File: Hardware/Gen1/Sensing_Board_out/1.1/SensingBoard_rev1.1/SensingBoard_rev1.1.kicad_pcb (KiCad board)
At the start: 6 copper layers, 40 x 40 mm, 89 parts, among them J1 USB_C_Receptacle, J2 3221-10-0300-00, J3 F32R-1A7H1-11024, J5 RS1-02-G, J6 RS1-02-G, J7 RS1-02-G, J9 RS1-02-G, SW1 PTS815 SJM 250 SMTR LFS, SW2 PTS815 SJM 250 SMTR LFS, U2 BNO055, U3 MIC5504-3.3YM5, U4 FT232RQ, U5 MIC5504-1.8YM5, U6 MCP1700x-280xxTT, U7 ESP32-S3, U8 GD25D05CT, Y1 ABM8G-40.000MHZ-18-D2Y-T

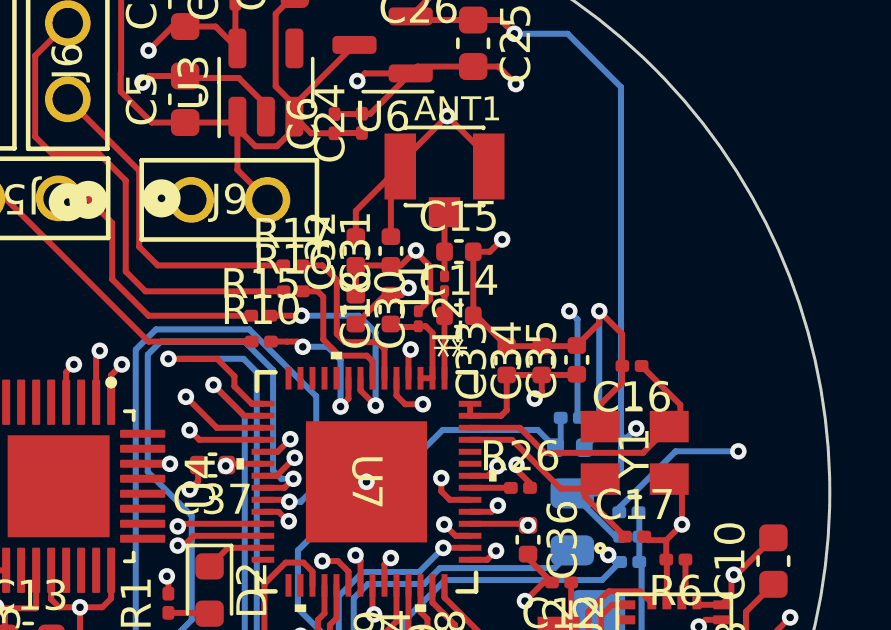
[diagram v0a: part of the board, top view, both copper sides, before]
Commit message: update
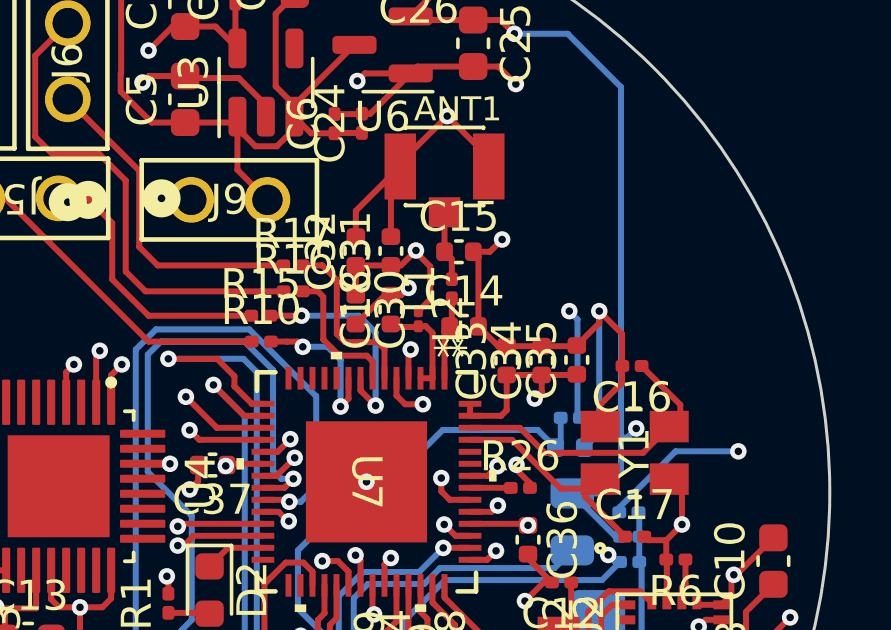
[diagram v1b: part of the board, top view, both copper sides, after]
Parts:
- L1: footprint Inductor_SMD:L_01005_0402Metric -> Inductor_SMD:L_0201_0603Metric
- moved C14 0.39 mm to (138.0, 56.9)
- moved L1 0.30 mm to (137.6, 55.7)

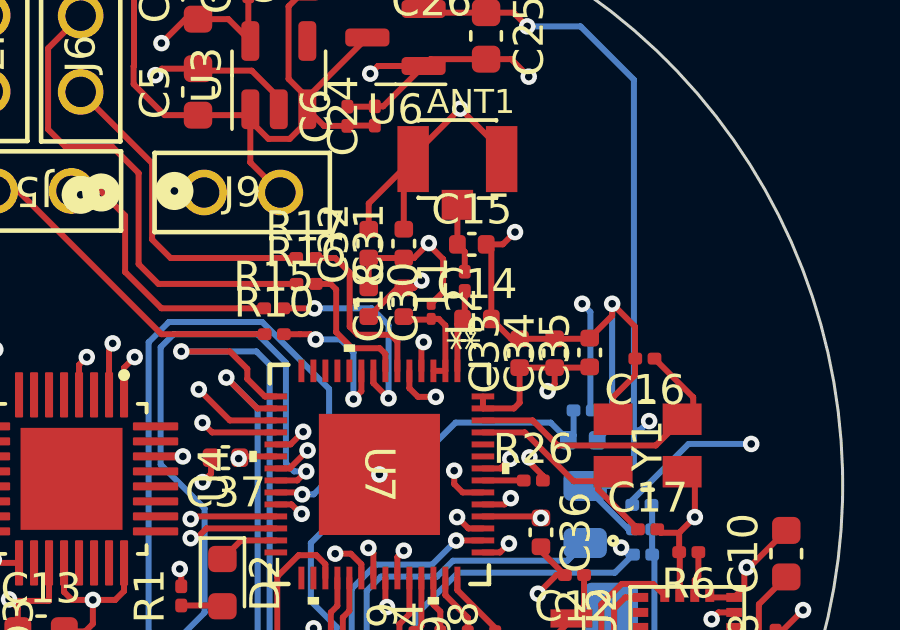
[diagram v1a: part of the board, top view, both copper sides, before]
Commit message: updates
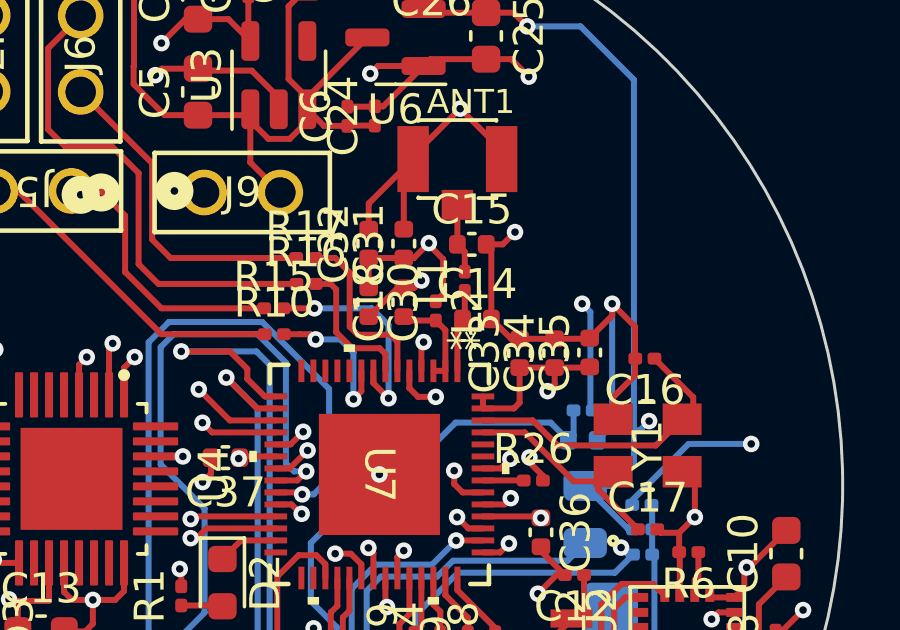
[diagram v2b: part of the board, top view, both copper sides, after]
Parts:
- L2: footprint Inductor_SMD:L_01005_0402Metric -> Inductor_SMD:L_0201_0603Metric
- moved L2 0.15 mm to (136.6, 56.7)
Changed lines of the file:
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@@
     (tags "ESP32-S3 ")
     (property "Mfr" "Espressif Systems")
-    (property "Mfr P/N" "ESP32-S3-WROOM-1-N8R2")
+    (property "Mfr P/N" "ESP32-S3R8")
     (property "Note" "")
     (property "Price" "4.3420")
-    (property "Purchase-URL" "https://www.lcsc.com/product-detail/WiFi-Modules_Espressif-Systems-ESP32-S3-WROOM-1-N8R2_C2913204.html")
+    (property "Purchase-URL" "https://www.lcsc.com/product-detail/RF-Transceiver-ICs_Espressif-Systems-ESP32-S3R8_C2913194.html")
     (property "Sheetfile" "SensingBoard_rev1.1.kicad_sch")
     (property "Sheetname" "")
     (property "Supplier 1" "LCSC")
-    (property "Supplier 1 P/N" "C2913204")
+    (property "Supplier 1 P/N" "C2913194")
     (property "ki_keywords" "ESP32-S3")
     (attr smd)
@@
         (effects (font (size 1 1) (thickness 0.15)))
     )
-    (fp_text user "*" (at -3.075001 -2.8 -90) (layer "F.Fab")
+    (fp_text user "*" (at -3.075001 -2.8 -90 unlocked) (layer "F.Fab")
         (effects (font (size 1 1) (thickness 0.15)))
     )
-    (fp_text user "*" (at -3.075001 -2.8 -90 unlocked) (layer "F.Fab")
+    (fp_text user "*" (at -3.075001 -2.8 -90) (layer "F.Fab")
         (effects (font (size 1 1) (thickness 0.15)))
     )
@@
     )
   )
-  (footprint "Inductor_SMD:L_01005_0402Metric" (layer "F.Cu")
-    (at 136.4488 56.6928 -90)
-    (descr "Inductor SMD 01005 (0402 Metric), square (rectangular) end terminal, IPC_7351 nominal, (Body size source: http://www.vishay.com/docs/20056/crcw01005e3.pdf), generated with kicad-footprint-generator")
+  (footprint "Inductor_SMD:L_0201_0603Metric" (layer "F.Cu")
+    (at 136.6012 56.6776 -90)
+    (descr "Inductor SMD 0201 (0603 Metric), square (rectangular) end terminal, IPC_7351 nominal, (Body size source: https://www.vishay.com/docs/20052/crcw0201e3.pdf), generated with kicad-footprint-generator")
     (tags "inductor")
     (property "Mfr" "Murata Electronics")
@@
     (property "ki_keywords" "inductor choke coil reactor magnetic")
     (attr smd)
-    (fp_text reference "L2" (at 0 -1 90) (layer "F.SilkS")
+    (fp_text reference "L2" (at 0 -1.05 -90) (layer "F.SilkS")
         (effects (font (size 1 1) (thickness 0.15)))
     )
-    (fp_text value "2nH" (at 0 1 90) (layer "F.Fab")
+    (fp_text value "2nH" (at 0 1.05 -90) (layer "F.Fab")
         (effects (font (size 1 1) (thickness 0.15)))
     )
-    (fp_text user "${REFERENCE}" (at 0 -0.62 90) (layer "F.Fab")
+    (fp_text user "${REFERENCE}" (at 0 -0.68 -90) (layer "F.Fab")
         (effects (font (size 0.25 0.25) (thickness 0.04)))
     )
-    (fp_line (start -0.6 -0.3) (end 0.6 -0.3)
+    (fp_line (start -0.7 -0.35) (end 0.7 -0.35)
       (stroke (width 0.05) (type solid)) (layer "F.CrtYd"))
-    (fp_line (start -0.6 0.3) (end -0.6 -0.3)
+    (fp_line (start -0.7 0.35) (end -0.7 -0.35)
       (stroke (width 0.05) (type solid)) (layer "F.CrtYd"))
-    (fp_line (start 0.6 -0.3) (end 0.6 0.3)
+    (fp_line (start 0.7 -0.35) (end 0.7 0.35)
       (stroke (width 0.05) (type solid)) (layer "F.CrtYd"))
-    (fp_line (start 0.6 0.3) (end -0.6 0.3)
+    (fp_line (start 0.7 0.35) (end -0.7 0.35)
       (stroke (width 0.05) (type solid)) (layer "F.CrtYd"))
-    (fp_line (start -0.2 -0.1) (end 0.2 -0.1)
+    (fp_line (start -0.3 -0.15) (end 0.3 -0.15)
       (stroke (width 0.1) (type solid)) (layer "F.Fab"))
-    (fp_line (start -0.2 0.1) (end -0.2 -0.1)
+    (fp_line (start -0.3 0.15) (end -0.3 -0.15)
       (stroke (width 0.1) (type solid)) (layer "F.Fab"))
-    (fp_line (start 0.2 -0.1) (end 0.2 0.1)
+    (fp_line (start 0.3 -0.15) (end 0.3 0.15)
       (stroke (width 0.1) (type solid)) (layer "F.Fab"))
-    (fp_line (start 0.2 0.1) (end -0.2 0.1)
+    (fp_line (start 0.3 0.15) (end -0.3 0.15)
       (stroke (width 0.1) (type solid)) (layer "F.Fab"))
-    (pad "" smd roundrect (at -0.275 0 270) (size 0.27 0.27) (layers "F.Paste") (roundrect_rratio 0.25))
-    (pad "" smd roundrect (at 0.275 0 270) (size 0.27 0.27) (layers "F.Paste") (roundrect_rratio 0.25))
-    (pad "1" smd roundrect (at -0.25 0 270) (size 0.4 0.3) (layers "F.Cu" "F.Mask") (roundrect_rratio 0.25)
+    (pad "" smd roundrect (at -0.345 0 270) (size 0.318 0.36) (layers "F.Paste") (roundrect_rratio 0.25))
+    (pad "" smd roundrect (at 0.345 0 270) (size 0.318 0.36) (layers "F.Paste") (roundrect_rratio 0.25))
+    (pad "1" smd roundrect (at -0.32 0 270) (size 0.46 0.4) (layers "F.Cu" "F.Mask") (roundrect_rratio 0.25)
       (net 69 "+3.3V") (pinfunction "1") (pintype "passive"))
-    (pad "2" smd roundrect (at 0.25 0 270) (size 0.4 0.3) (layers "F.Cu" "F.Mask") (roundrect_rratio 0.25)
+    (pad "2" smd roundrect (at 0.32 0 270) (size 0.46 0.4) (layers "F.Cu" "F.Mask") (roundrect_rratio 0.25)
       (net 16 "Net-(C18-Pad1)") (pinfunction "2") (pintype "passive"))
-    (model "${KICAD6_3DMODEL_DIR}/Inductor_SMD.3dshapes/L_01005_0402Metric.wrl"
+    (model "${KICAD6_3DMODEL_DIR}/Inductor_SMD.3dshapes/L_0201_0603Metric.wrl"
       (offset (xyz 0 0 0))
       (scale (xyz 1 1 1))
@@
   (segment (start 138.305297 47.932097) (end 136.1488 45.7756) (width 0.2) (layer "In4.Cu") (net 14))
   (segment (start 138.305297 66.423297) (end 138.305297 47.932097) (width 0.2) (layer "In4.Cu") (net 14))
-  (segment (start 135.6342 56.9678) (end 136.358115 56.9678) (width 0.2) (layer "F.Cu") (net 16))
-  (segment (start 136.6988 56.9428) (end 136.9216 57.1656) (width 0.2) (layer "F.Cu") (net 16))
+  (segment (start 136.921601 57.318001) (end 136.6012 56.9976) (width 0.2) (layer "F.Cu") (net 16))
+  (segment (start 136.6012 56.9976) (end 135.664 56.9976) (width 0.2) (layer "F.Cu") (net 16))
+  (segment (start 136.921601 58.675999) (end 136.921601 57.318001) (width 0.2) (layer "F.Cu") (net 16))
+  (segment (start 135.664 56.9976) (end 135.5344 56.868) (width 0.2) (layer "F.Cu") (net 16))
   (segment (start 136.921601 58.675999) (end 136.521599 58.675999) (width 0.2) (layer "F.Cu") (net 16))
-  (segment (start 135.5344 56.868) (end 135.6342 56.9678) (width 0.2) (layer "F.Cu") (net 16))
-  (segment (start 136.4488 56.9428) (end 136.6988 56.9428) (width 0.2) (layer "F.Cu") (net 16))
-  (segment (start 136.9216 57.1656) (end 136.921601 58.675999) (width 0.2) (layer "F.Cu") (net 16))
   (segment (start 116.4488 52.7613) (end 116.4488 51.1782) (width 0.2) (layer "F.Cu") (net 17))
   (segment (start 116.4488 52.7613) (end 117.1249 52.7613) (width 0.2) (layer "F.Cu") (net 17))
@@
   (segment (start 118.3132 72.0344) (end 118.872 72.5932) (width 0.2) (layer "B.Cu") (net 68))
   (segment (start 135.6168 73.406) (end 135.2992 73.0884) (width 0.2) (layer "B.Cu") (net 68))
+  (segment (start 136.6012 56.3576) (end 136.847001 56.111799) (width 0.2) (layer "F.Cu") (net 69))
   (segment (start 136.7536 75.8672) (end 136.7536 76.2) (width 0.2) (layer "F.Cu") (net 69))
   (segment (start 144.7332 70.7909) (end 144.7332 70.3528) (width 0.2) (layer "F.Cu") (net 69))
   (segment (start 130.3528 47.6153) (end 130.4188 47.6813) (width 0.2) (layer "F.Cu") (net 69))
   (segment (start 136.369675 54.417709) (end 136.369675 54.474882) (width 0.2) (layer "F.Cu") (net 69))
-  (segment (start 136.847001 54.952208) (end 136.847001 56.044599) (width 0.2) (layer "F.Cu") (net 69))
   (segment (start 139.3952 58.5672) (end 140.5636 58.5672) (width 0.2) (layer "F.Cu") (net 69))
   (segment (start 135.1026 75.3198) (end 135.65 75.8672) (width 0.2) (layer "F.Cu") (net 69))
@@
   (segment (start 141.3514 71.9578) (end 140.97 72.3392) (width 0.2) (layer "F.Cu") (net 69))
   (segment (start 142.8582 70.2284) (end 142.1642 70.9224) (width 0.2) (layer "F.Cu") (net 69))
+  (segment (start 136.847001 56.111799) (end 136.847001 54.952208) (width 0.2) (layer "F.Cu") (net 69))
   (segment (start 134.366 54.9148) (end 135.5344 54.9148) (width 0.2) (layer "F.Cu") (net 69))
   (segment (start 133.3962 81.28) (end 132.4864 81.28) (width 0.2) (layer "F.Cu") (net 69))
@@
   (segment (start 126.21 58.5726) (end 126.21 59.8268) (width 0.2) (layer "F.Cu") (net 69))
   (segment (start 136.940112 72.2884) (end 136.519984 72.708528) (width 0.2) (layer "F.Cu") (net 69))
-  (segment (start 136.4738 56.4178) (end 136.4488 56.4178) (width 0.2) (layer "F.Cu") (net 69))
   (segment (start 120.8532 74.702796) (end 120.8532 76.3524) (width 0.2) (layer "F.Cu") (net 69))
   (segment (start 144.7332 70.7909) (end 145.2332 70.7909) (width 0.2) (layer "F.Cu") (net 69))
@@
   (segment (start 138.174001 59.5284) (end 138.174001 59.928399) (width 0.2) (layer "F.Cu") (net 69))
   (segment (start 130.3528 46.1924) (end 130.3528 47.6153) (width 0.2) (layer "F.Cu") (net 69))
-  (segment (start 136.847001 56.044599) (end 136.4738 56.4178) (width 0.2) (layer "F.Cu") (net 69))
   (segment (start 137.734 69.6468) (end 138.4854 69.6468) (width 0.2) (layer "F.Cu") (net 69))
   (via (at 122.3772 66.294) (size 0.55) (drill 0.25) (layers "F.Cu" "B.Cu") (net 69))
